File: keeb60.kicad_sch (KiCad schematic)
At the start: 1 part, among them U1 nice_nano

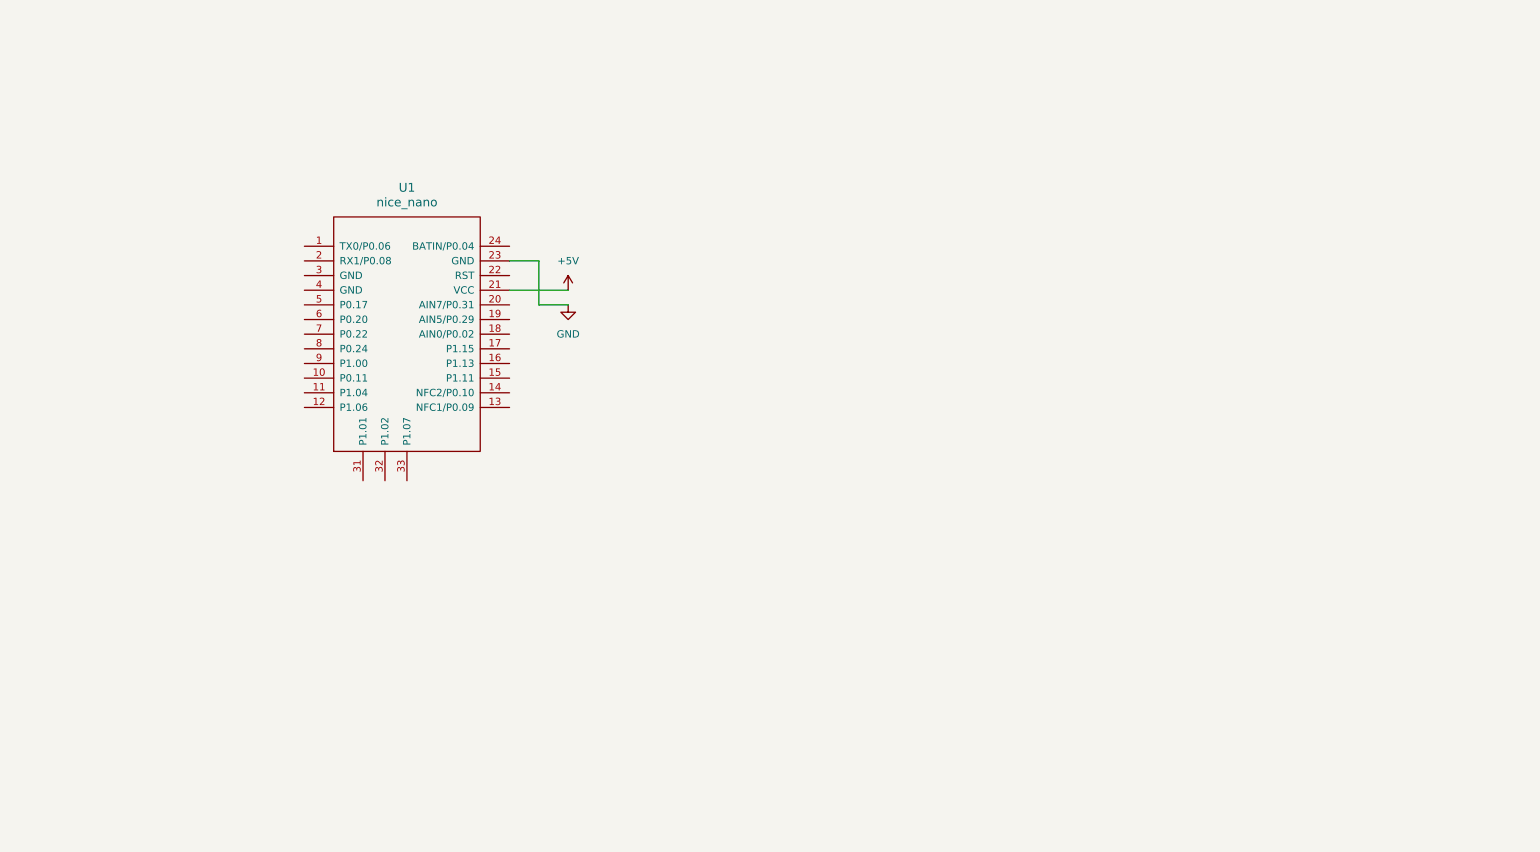
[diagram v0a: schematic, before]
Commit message: Add matrix
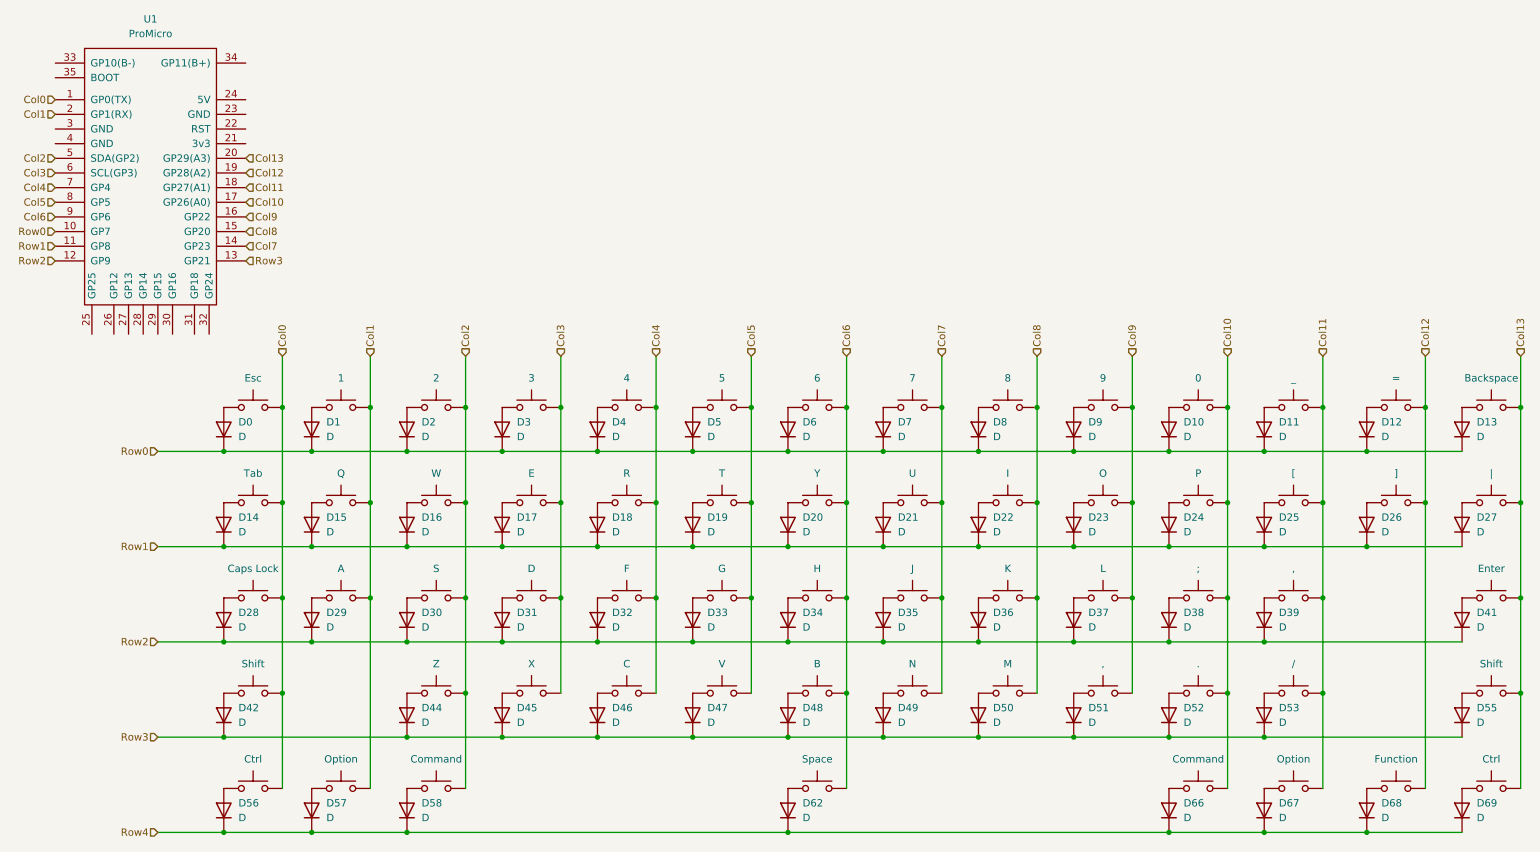
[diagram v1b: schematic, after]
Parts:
- removed U1: nice_nano, symbol nice_nano:nice_nano
- added D0, D1, D10, D11, D12, D13, D14, D15, D16, D17, D18, D19, D2, D20, D21, D22, D23, D24, D25, D26, D27, D28, D29, D3, D30, D31, D32, D33, D34, D35, D36, D37, D38, D39, D4, D41, D42, D44, D45, D46, D47, D48, D49, D5, D50, D51, D52, D53, D55, D56, D57, D58, D6, D62, D66, D67, D68, D69, D7, D8, D9: D, symbol Device:D
- added K000: Esc, symbol Switch:SW_Push
- added K001: 1, symbol Switch:SW_Push
- added K002: 2, symbol Switch:SW_Push
- added K003: 3, symbol Switch:SW_Push
- added K004: 4, symbol Switch:SW_Push
- added K005: 5, symbol Switch:SW_Push
- added K006: 6, symbol Switch:SW_Push
- added K007: 7, symbol Switch:SW_Push
- added K008: 8, symbol Switch:SW_Push
- added K009: 9, symbol Switch:SW_Push
- added K010: 0, symbol Switch:SW_Push
- added K011: _, symbol Switch:SW_Push
- added K012: =, symbol Switch:SW_Push
- added K013: Backspace, symbol Switch:SW_Push
- added K100: Tab, symbol Switch:SW_Push
- added K101: Q, symbol Switch:SW_Push
- added K102: W, symbol Switch:SW_Push
- added K103: E, symbol Switch:SW_Push
- added K104: R, symbol Switch:SW_Push
- added K105: T, symbol Switch:SW_Push
- added K106: Y, symbol Switch:SW_Push
- added K107: U, symbol Switch:SW_Push
- added K108: I, symbol Switch:SW_Push
- added K109: O, symbol Switch:SW_Push
- added K110: P, symbol Switch:SW_Push
- added K111: [, symbol Switch:SW_Push
- added K112: ], symbol Switch:SW_Push
- added K113: |, symbol Switch:SW_Push
- added K200: Caps Lock, symbol Switch:SW_Push
- added K201: A, symbol Switch:SW_Push
- added K202: S, symbol Switch:SW_Push
- added K203: D, symbol Switch:SW_Push
- added K204: F, symbol Switch:SW_Push
- added K205: G, symbol Switch:SW_Push
- added K206: H, symbol Switch:SW_Push
- added K207: J, symbol Switch:SW_Push
- added K208: K, symbol Switch:SW_Push
- added K209: L, symbol Switch:SW_Push
- added K210: ;, symbol Switch:SW_Push
- added K211, K309: ,, symbol Switch:SW_Push
- added K213: Enter, symbol Switch:SW_Push
- added K300, K313: Shift, symbol Switch:SW_Push
- added K302: Z, symbol Switch:SW_Push
- added K303: X, symbol Switch:SW_Push
- added K304: C, symbol Switch:SW_Push
- added K305: V, symbol Switch:SW_Push
- added K306: B, symbol Switch:SW_Push
- added K307: N, symbol Switch:SW_Push
- added K308: M, symbol Switch:SW_Push
- added K310: ., symbol Switch:SW_Push
- added K311: /, symbol Switch:SW_Push
- added K400, K413: Ctrl, symbol Switch:SW_Push
- added K401, K411: Option, symbol Switch:SW_Push
- added K402, K410: Command, symbol Switch:SW_Push
- added K406: Space, symbol Switch:SW_Push
- added K412: Function, symbol Switch:SW_Push
- added U1: ProMicro, Zodiark:ProMicro_rev2, symbol TheOneProMicro:ProMicro_2-Lily58-cache
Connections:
- new net: D41.2 (A), K213.1
- new net: D15.2 (A), K101.1
- new net: D44.2 (A), K302.1
- new net: D55.2 (A), K313.1
- new net: D45.2 (A), K303.1
- new net: D46.2 (A), K304.1
- new net: D42.2 (A), K300.1
- new net: D30.2 (A), K202.1
- new net: D34.2 (A), K206.1
- new net: D16.2 (A), K102.1
- new net: D4.2 (A), K004.1
- new net: D51.2 (A), K309.1
- new net: D3.2 (A), K003.1
- new net: D67.2 (A), K411.1
- new net: D36.2 (A), K208.1
- new net: D58.2 (A), K402.1
- new net: D62.2 (A), K406.1
- new net: D49.2 (A), K307.1
- new net: D12.2 (A), K012.1
- new net: D28.2 (A), K200.1
- new net: D9.2 (A), K009.1
- new net: D31.2 (A), K203.1
- new net: D57.2 (A), K401.1
- new net: D32.2 (A), K204.1
- new net: D0.2 (A), K000.1
- new net: D66.2 (A), K410.1
- new net: D11.2 (A), K011.1
- new net: D10.2 (A), K010.1
- new net: D8.2 (A), K008.1
- new net: D6.2 (A), K006.1
- new net: D18.2 (A), K104.1
- new net: D47.2 (A), K305.1
- new net: D24.2 (A), K110.1
- new net: D7.2 (A), K007.1
- new net: D52.2 (A), K310.1
- new net: D22.2 (A), K108.1
- new net: D19.2 (A), K105.1
- new net: D68.2 (A), K412.1
- new net: D29.2 (A), K201.1
- new net: D53.2 (A), K311.1
- new net: D26.2 (A), K112.1
- new net: D27.2 (A), K113.1
- new net: D14.2 (A), K100.1
- new net: D17.2 (A), K103.1
- new net: D39.2 (A), K211.1
- new net: D37.2 (A), K209.1
- new net: D2.2 (A), K002.1
- new net: D21.2 (A), K107.1
- new net: D5.2 (A), K005.1
- new net: D56.2 (A), K400.1
- new net: D48.2 (A), K306.1
- new net: D25.2 (A), K111.1
- new net: D20.2 (A), K106.1
- new net: D33.2 (A), K205.1
- new net: D35.2 (A), K207.1
- new net: D23.2 (A), K109.1
- new net: D38.2 (A), K210.1
- new net: D13.2 (A), K013.1
- new net: D50.2 (A), K308.1
- new net: D1.2 (A), K001.1
- new net: D69.2 (A), K413.1
- new net Col0: K000.2, K100.2, K200.2, K300.2, K400.2, U1.1 (GP0(TX))
- new net Col1: K001.2, K101.2, K201.2, K401.2, U1.2 (GP1(RX))
- new net Col10: K010.2, K110.2, K210.2, K310.2, K410.2, U1.17 (GP26(A0))
- new net Col11: K011.2, K111.2, K211.2, K311.2, K411.2, U1.18 (GP27(A1))
- new net Col12: K012.2, K112.2, K412.2, U1.19 (GP28(A2))
- new net Col13: K013.2, K113.2, K213.2, K313.2, K413.2, U1.20 (GP29(A3))
- new net Col2: K002.2, K102.2, K202.2, K302.2, K402.2, U1.5 (SDA(GP2))
- new net Col3: K003.2, K103.2, K203.2, K303.2, U1.6 (SCL(GP3))
- new net Col4: K004.2, K104.2, K204.2, K304.2, U1.7 (GP4)
- new net Col5: K005.2, K105.2, K205.2, K305.2, U1.8 (GP5)
- new net Col6: K006.2, K106.2, K206.2, K306.2, K406.2, U1.9 (GP6)
- new net Col7: K007.2, K107.2, K207.2, K307.2, U1.14 (GP23)
- new net Col8: K008.2, K108.2, K208.2, K308.2, U1.15 (GP20)
- new net Col9: K009.2, K109.2, K209.2, K309.2, U1.16 (GP22)
- new net Row0: D0.1 (K), D1.1 (K), D10.1 (K), D11.1 (K), D12.1 (K), D13.1 (K), D2.1 (K), D3.1 (K), D4.1 (K), D5.1 (K), D6.1 (K), D7.1 (K), D8.1 (K), D9.1 (K), U1.10 (GP7)
- new net Row1: D14.1 (K), D15.1 (K), D16.1 (K), D17.1 (K), D18.1 (K), D19.1 (K), D20.1 (K), D21.1 (K), D22.1 (K), D23.1 (K), D24.1 (K), D25.1 (K), D26.1 (K), D27.1 (K), U1.11 (GP8)
- new net Row2: D28.1 (K), D29.1 (K), D30.1 (K), D31.1 (K), D32.1 (K), D33.1 (K), D34.1 (K), D35.1 (K), D36.1 (K), D37.1 (K), D38.1 (K), D39.1 (K), D41.1 (K), U1.12 (GP9)
- new net Row3: D42.1 (K), D44.1 (K), D45.1 (K), D46.1 (K), D47.1 (K), D48.1 (K), D49.1 (K), D50.1 (K), D51.1 (K), D52.1 (K), D53.1 (K), D55.1 (K), U1.13 (GP21)
- new net Row4: D56.1 (K), D57.1 (K), D58.1 (K), D62.1 (K), D66.1 (K), D67.1 (K), D68.1 (K), D69.1 (K)
